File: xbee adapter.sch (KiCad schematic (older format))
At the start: 12 parts, among them P1 CONN_10, P2 CONN_10, U1 LM1117-3.3, U2 XBEE

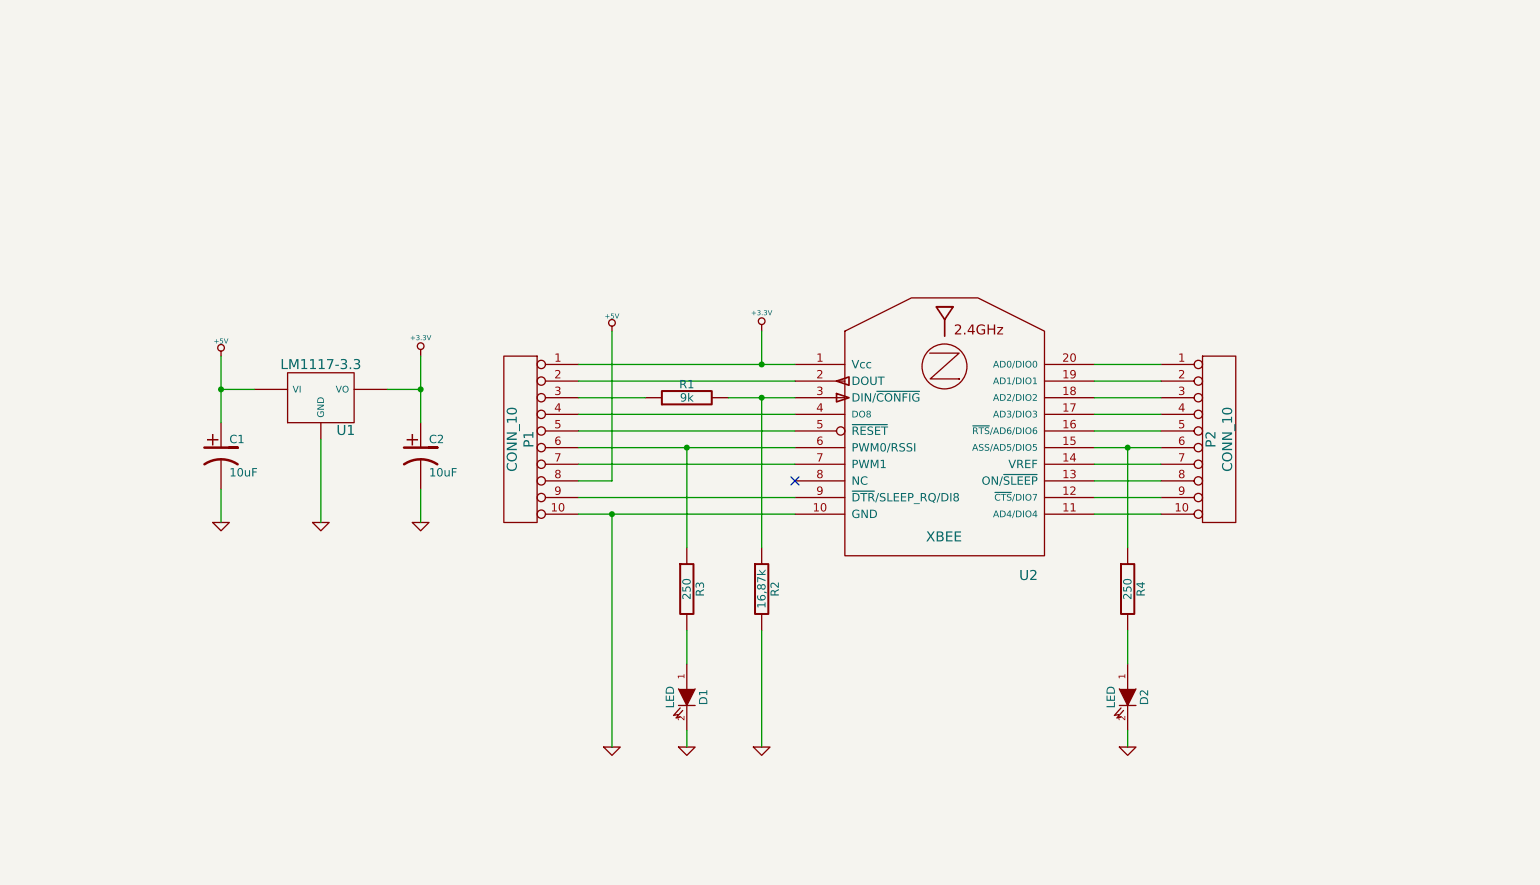
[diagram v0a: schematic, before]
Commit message: [XBEE] agrego archivos faltantes
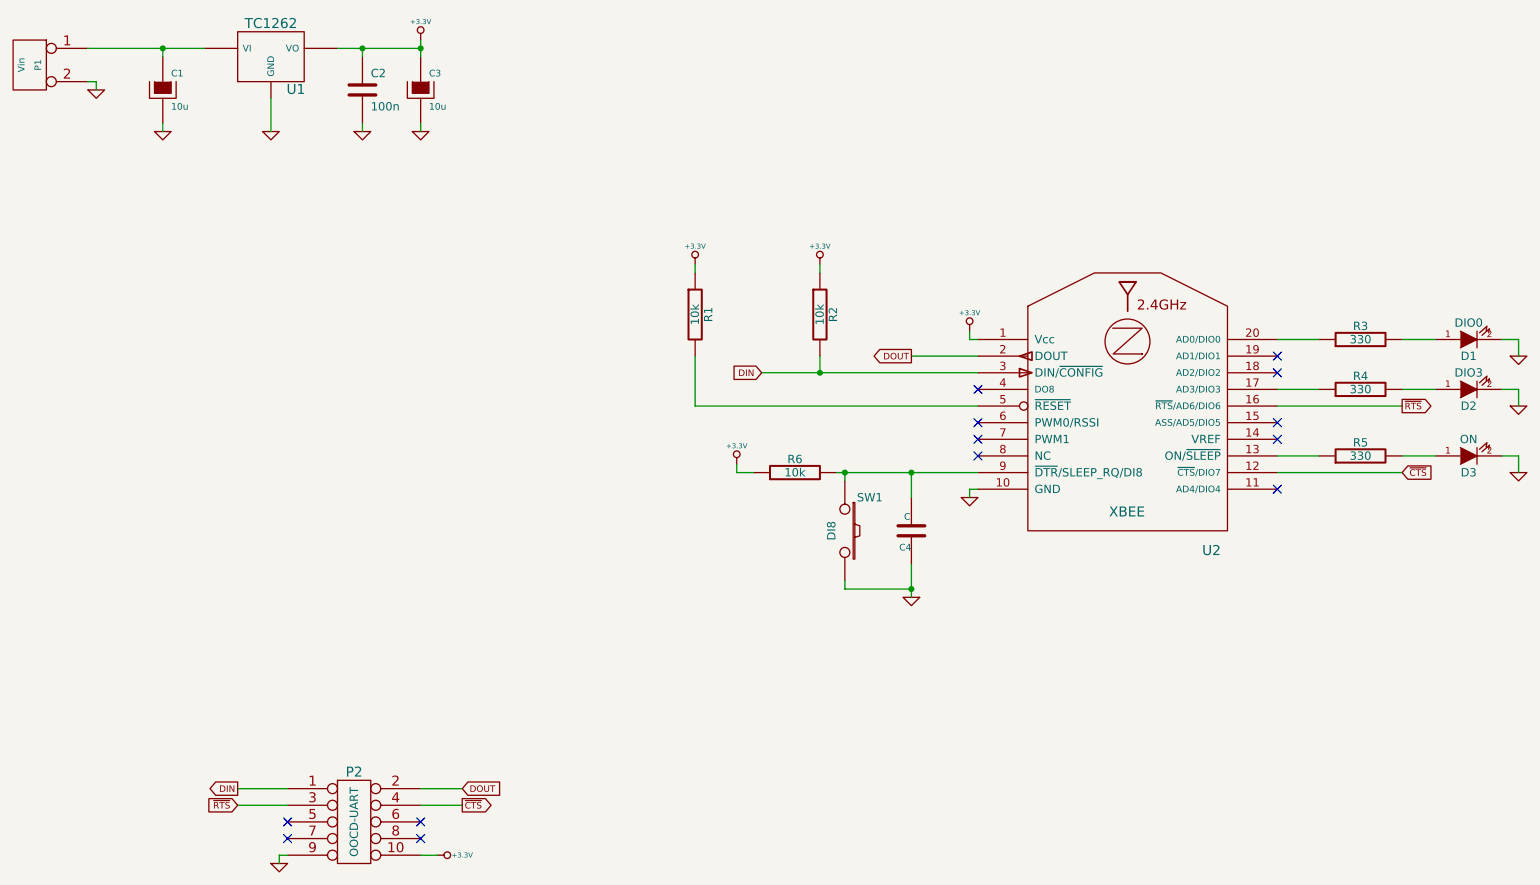
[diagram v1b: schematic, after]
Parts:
- removed C1, C2: 10uF, symbol CP1
- removed D1: LED, symbol LED
- removed P1, P2: CONN_10, symbol CONN_10
- removed R3: 250, symbol R
- removed U1: LM1117-3.3, symbol LM1117-3.3
- added C1, C3: 10u, ~, symbol CAPAPOL
- added C2: 100n, symbol C
- added C4: C, ~, symbol C
- added D2: DIO3, symbol LED
- added D3: ON, symbol LED
- added P1: Vin, symbol CONN_2
- added P2: OOCD-UART, symbol CONN_5X2
- added R4, R5: 330, symbol R
- added R6: 10k, symbol R
- added SW1: DI8, ~, symbol SW_PUSH
- added U1: TC1262, symbol TC1262
- D1: renamed from D2; value LED -> DIO0
- R1: value 9k -> 10k
- R2: value 16,87k -> 10k
- R3: renamed from R4; value 250 -> 330
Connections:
- net +3.3V: now also R1.1, R2.1, C2.1, C3.1, P2.10, R6.1, U1.3 (VO)
- net GND: now also C1.2, C2.2, C3.2, C4.1, D2.2 (K), D3.2 (K), P1.2 (PM), P2.9, SW1.2, U1.2 (GND); no longer R2.2
- net ~CTS: now reaches U2.12 (~CTS~/DIO7)
- net ~CTS: now also P2.4
- net at U2.13 (ON/~SLEEP): now also R5.1
- net at U2.15 (ASS/AD5/DIO5): no longer R3.1
- net ~RTS: now reaches U2.16 (~RTS~/AD6/DIO6)
- net ~RTS: now also P2.3
- net at U2.17 (AD3/DIO3): now also R4.1
- net DOUT: now reaches U2.2 (DOUT)
- net DOUT: now also P2.2
- net at U2.20 (AD0/DIO0): now also R3.1
- net at U2.5 (~RESET): now also R1.2
- net at U2.9 (~DTR~/SLEEP_RQ/DI8): now also C4.2, R6.2, SW1.1
- new net: D2.1 (A), R4.2
- new net: D3.1 (A), R5.2
- new net: C1.1, P1.1 (P1), U1.1 (VI)
- new net DIN: P2.1, R2.2, U2.3 (DIN/~CONFIG)
- no-connect marks 1 -> 13
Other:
- moved on the sheet: D1, R3, U2
